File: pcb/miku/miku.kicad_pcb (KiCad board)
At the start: 2 copper layers, 71.1 x 108 mm, 25 parts, among them J01 MIDI_IN, J02 PITCH_CV_IN, J03 GATE_IN, J04 VOL_CV_IN, J05 SYLL_CV_IN, J06 PORT_CV_IN, J07 TBD_IN, J08 VIBTYPE_CV_IN, J09 VIBRATE_CV_IN, J10 VIBDELAY_CV_IN, J11 AUDIO_L_OUT, J12 AUDIO_R_ROUT

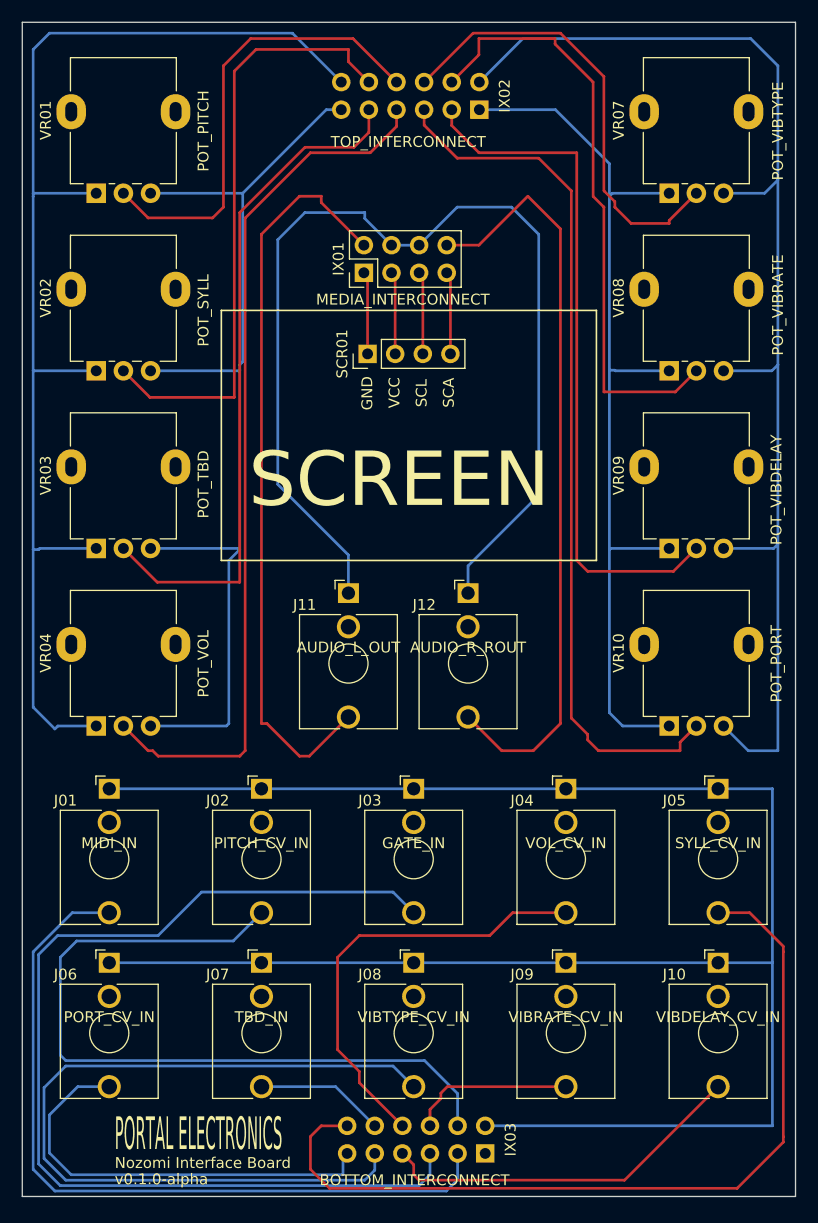
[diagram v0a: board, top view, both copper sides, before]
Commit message: Silkscreened the IX pinouts
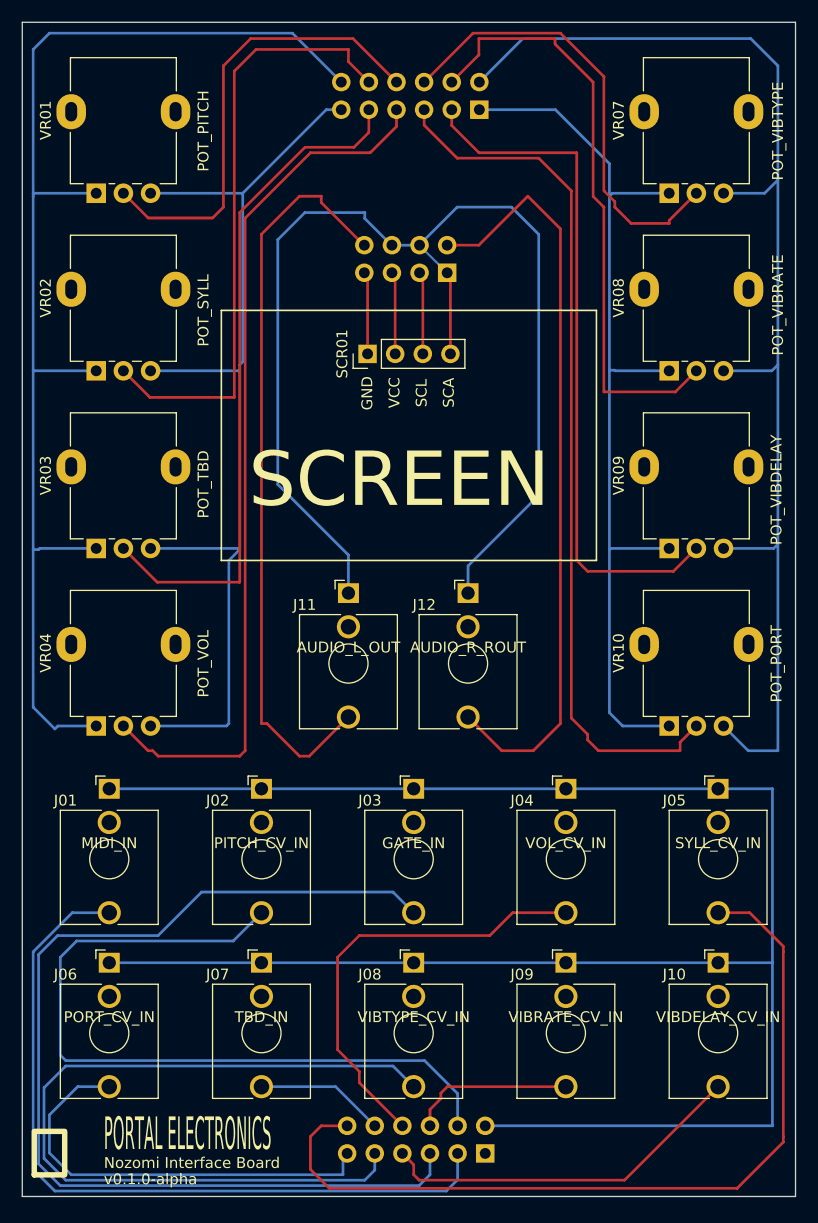
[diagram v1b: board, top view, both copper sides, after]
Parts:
- IX01: renamed from IX02; value TOP_INTERCONNECT -> TOP_IX
- IX02: renamed from IX01; value MEDIA_INTERCONNECT -> MEDIA_IX; moved to B.Cu
- IX03: value BOTTOM_INTERCONNECT -> BOTTOM_IX
- moved IX02 7.66 mm to (114.1, 62.5)
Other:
- board text added: "3.3VA"
- board text added: "AUDL"
- board text added: "AUDR"
- board text added: "PITCH"
- board text added: "PORTM"
- board text added: "SCRN"
- board text added: "SYLL"
- board text added: "VIBDL"
- board text added: "VIBRT"
- board text added: "VIBTP"
- board text added: "VOLUM"
- board text added: "望"

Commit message: Revert "Added silkscreen labels for interconnect pins (#30)"
This reverts commit c19aa1e4f3f042fac9955cee06975aab86f3ba47.
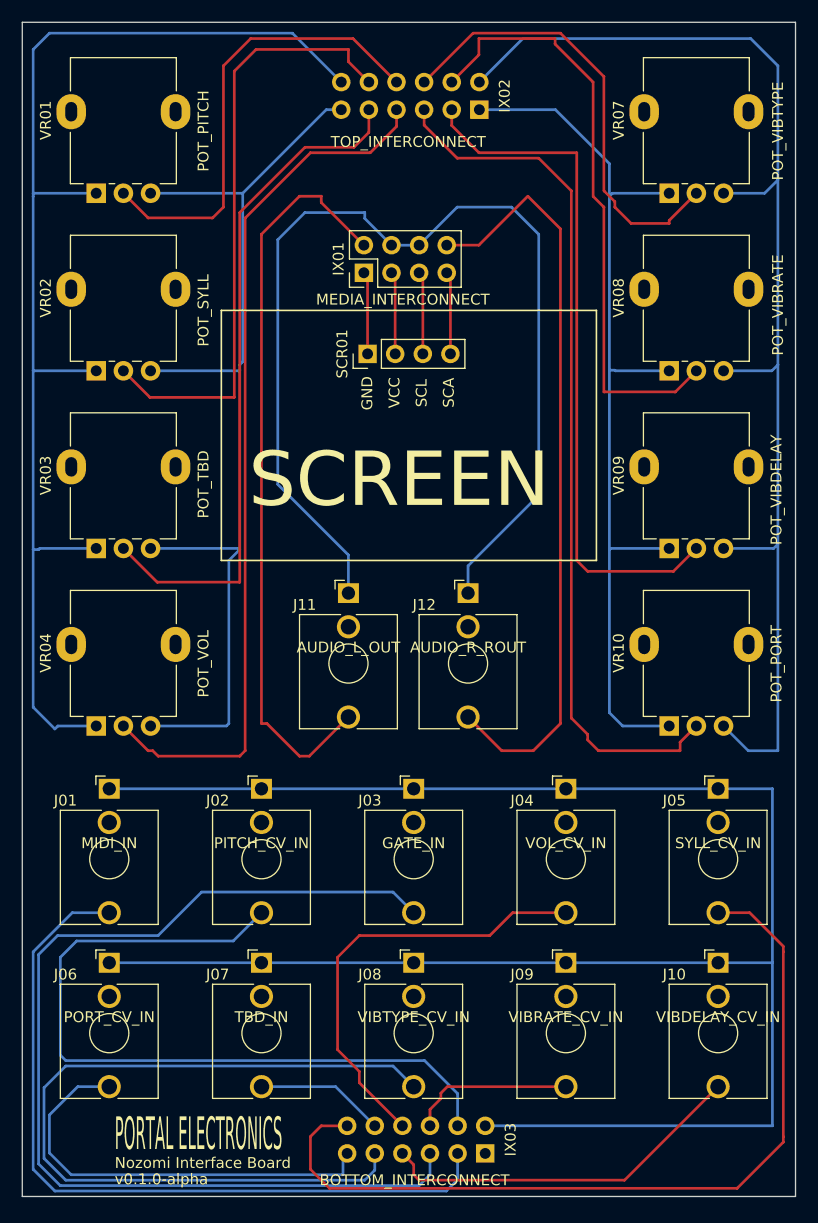
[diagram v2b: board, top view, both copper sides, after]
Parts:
- IX01: renamed from IX02; value MEDIA_IX -> MEDIA_INTERCONNECT; moved to F.Cu
- IX02: renamed from IX01; value TOP_IX -> TOP_INTERCONNECT
- IX03: value BOTTOM_IX -> BOTTOM_INTERCONNECT
- moved IX01 7.66 mm to (106.4, 62.5)
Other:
- board text removed: "3.3VA"
- board text removed: "AUDL"
- board text removed: "AUDR"
- board text removed: "PITCH"
- board text removed: "PORTM"
- board text removed: "SCRN"
- board text removed: "SYLL"
- board text removed: "VIBDL"
- board text removed: "VIBRT"
- board text removed: "VIBTP"
- board text removed: "VOLUM"
- board text removed: "望"
